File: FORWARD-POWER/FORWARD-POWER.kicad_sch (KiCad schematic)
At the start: 17 parts, among them J1 Conn_01x03_Pin, J2 Conn_01x03_Pin, J4 Screw_Terminal_01x04, U2 AMS1117-5.0, U3 AMS1117-3.3

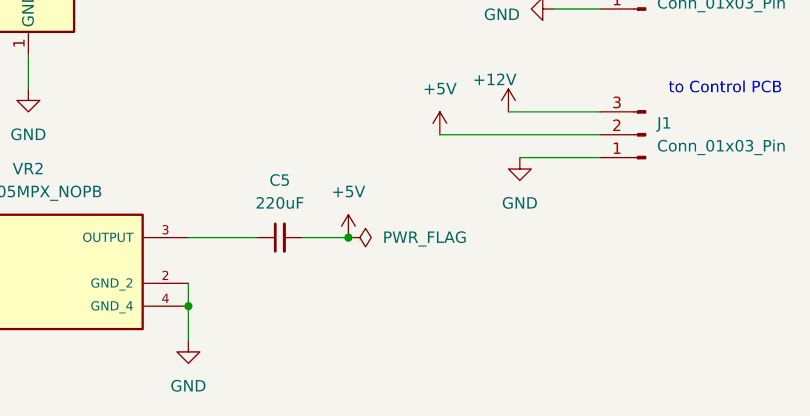
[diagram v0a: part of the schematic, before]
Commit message: ready to order (i think)
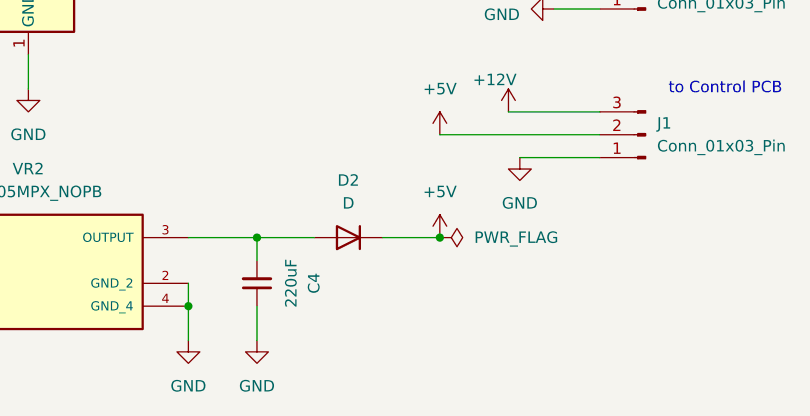
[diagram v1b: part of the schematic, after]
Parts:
- removed C5: 220uF, Capacitor_SMD:C_0805_2012Metric, symbol Device:C_Small
- added C4: 220uF, Capacitor_SMD:C_0805_2012Metric, symbol Device:C_Small
- added D2: D, Diode_SMD:D_0805_2012Metric, symbol Device:D
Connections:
- net +5V: now also D2.1 (K)
- net GND: now also C4.1
- net at VR2.3 (OUTPUT): now also C4.2, D2.2 (A)
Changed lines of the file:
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@@
+	)
+	(junction
+		(at 163.83 142.24)
+		(diameter 0)
+		(color 0 0 0 0)
 	)
 	(junction
@@
 	)
 	(junction
-		(at 173.99 142.24)
+		(at 184.15 142.24)
 		(diameter 0)
 		(color 0 0 0 0)
@@
 	(wire
 		(pts
-			(xy 173.99 142.24) (xy 168.91 142.24)
-		)
-		(stroke
-			(width 0)
-			(type default)
-		)
-	)
-	(wire
-		(pts
 			(xy 90.17 124.46) (xy 90.17 127)
 		)
@@
 	(wire
 		(pts
+			(xy 177.8 142.24) (xy 184.15 142.24)
+		)
+		(stroke
+			(width 0)
+			(type default)
+		)
+	)
+	(wire
+		(pts
 			(xy 123.19 72.39) (xy 132.08 72.39)
 		)
@@
 	(wire
 		(pts
+			(xy 163.83 142.24) (xy 163.83 144.78)
+		)
+		(stroke
+			(width 0)
+			(type default)
+		)
+	)
+	(wire
+		(pts
 			(xy 132.08 72.39) (xy 132.08 81.28)
 		)
@@
 	(wire
 		(pts
+			(xy 163.83 153.67) (xy 163.83 149.86)
+		)
+		(stroke
+			(width 0)
+			(type default)
+		)
+	)
+	(wire
+		(pts
 			(xy 156.21 149.86) (xy 156.21 147.32)
 		)
@@
 		(pts
 			(xy 156.21 153.67) (xy 156.21 149.86)
+		)
+		(stroke
+			(width 0)
+			(type default)
+		)
+	)
+	(wire
+		(pts
+			(xy 163.83 142.24) (xy 170.18 142.24)
 		)
 		(stroke
@@
 	)
 	(symbol
+		(lib_id "Device:D")
+		(at 173.99 142.24 180)
+		(unit 1)
+		(exclude_from_sim no)
+		(in_bom yes)
+		(on_board yes)
+		(dnp no)
+		(fields_autoplaced yes)
+		(property "Reference" "D2"
+			(at 173.99 135.89 0)
+			(effects
+				(font
+					(size 1.27 1.27)
+				)
+			)
+		)
+		(property "Value" "D"
+			(at 173.99 138.43 0)
+			(effects
+				(font
+					(size 1.27 1.27)
+				)
+			)
+		)
+		(property "Footprint" "Diode_SMD:D_0805_2012Metric"
+			(at 173.99 142.24 0)
+			(effects
+				(font
+					(size 1.27 1.27)
+				)
+				(hide yes)
+			)
+		)
+		(property "Datasheet" "~"
+			(at 173.99 142.24 0)
+			(effects
+				(font
+					(size 1.27 1.27)
+				)
+				(hide yes)
+			)
+		)
+		(property "Description" "Diode"
+			(at 173.99 142.24 0)
+			(effects
+				(font
+					(size 1.27 1.27)
+				)
+				(hide yes)
+			)
+		)
+		(property "Sim.Device" "D"
+			(at 173.99 142.24 0)
+			(effects
+				(font
+					(size 1.27 1.27)
+				)
+				(hide yes)
+			)
+		)
+		(property "Sim.Pins" "1=K 2=A"
+			(at 173.99 142.24 0)
+			(effects
+				(font
+					(size 1.27 1.27)
+				)
+				(hide yes)
+			)
+		)
+		(pin "1"
+		)
+		(pin "2"
+		)
+		(instances
+			(project ""
+				(path "/ce51f21b-ae90-4513-bbba-00af99e3d46b"
+					(reference "D2")
+					(unit 1)
+				)
+			)
+		)
+	)
+	(symbol
 		(lib_id "power:+6V")
 		(at 85.09 123.19 0)
@@
 	(symbol
 		(lib_id "power:PWR_FLAG")
-		(at 173.99 142.24 270)
+		(at 184.15 142.24 270)
 		(unit 1)
 		(exclude_from_sim no)
@@
 		(fields_autoplaced yes)
 		(property "Reference" "#FLG03"
-			(at 175.895 142.24 0)
+			(at 186.055 142.24 0)
 			(effects
 				(font
@@
 		)
 		(property "Value" "PWR_FLAG"
-			(at 177.8 142.2399 90)
+			(at 187.96 142.2399 90)
 			(effects
 				(font
@@
 		)
 		(property "Footprint" ""
-			(at 173.99 142.24 0)
+			(at 184.15 142.24 0)
 			(effects
 				(font
@@
 		)
 		(property "Datasheet" "~"
-			(at 173.99 142.24 0)
+			(at 184.15 142.24 0)
 			(effects
 				(font
@@
 		)
 		(property "Description" "Special symbol for telling ERC where power comes from"
-			(at 173.99 142.24 0)
+			(at 184.15 142.24 0)
 			(effects
 				(font
@@
 	)
 	(symbol
-		(lib_id "Device:C_Small")
-		(at 166.37 142.24 90)
-		(unit 1)
-		(exclude_from_sim no)
-		(in_bom yes)
-		(on_board yes)
-		(dnp no)
-		(fields_autoplaced yes)
-		(property "Reference" "C5"
-			(at 166.3763 135.89 90)
-			(effects
-				(font
-					(size 1.27 1.27)
-				)
-			)
-		)
-		(property "Value" "220uF"
-			(at 166.3763 138.43 90)
-			(effects
-				(font
-					(size 1.27 1.27)
-				)
-			)
-		)
-		(property "Footprint" "Capacitor_SMD:C_0805_2012Metric"
-			(at 166.37 142.24 0)
-			(effects
-				(font
-					(size 1.27 1.27)
-				)
-				(hide yes)
-			)
-		)
-		(property "Datasheet" "~"
-			(at 166.37 142.24 0)
-			(effects
-				(font
-					(size 1.27 1.27)
-				)
-				(hide yes)
-			)
-		)
-		(property "Description" "Unpolarized capacitor, small symbol"
-			(at 166.37 142.24 0)
-			(effects
-				(font
-					(size 1.27 1.27)
-				)
-				(hide yes)
-			)
-		)
-		(pin "2"
-		)
-		(pin "1"
-		)
-		(instances
-			(project ""
-				(path "/ce51f21b-ae90-4513-bbba-00af99e3d46b"
-					(reference "C5")
-					(unit 1)
-				)
-			)
-		)
-	)
-	(symbol
 		(lib_id "power:+3.3V")
 		(at 196.85 111.76 90)
@@
 	)
 	(symbol
+		(lib_id "power:GND")
+		(at 163.83 153.67 0)
+		(unit 1)
+		(exclude_from_sim no)
+		(in_bom yes)
+		(on_board yes)
+		(dnp no)
+		(fields_autoplaced yes)
+		(property "Reference" "#PWR06"
+			(at 163.83 160.02 0)
+			(effects
+				(font
+					(size 1.27 1.27)
+				)
+				(hide yes)
+			)
+		)
+		(property "Value" "GND"
+			(at 163.83 158.75 0)
+			(effects
+				(font
+					(size 1.27 1.27)
+				)
+			)
+		)
+		(property "Footprint" ""
+			(at 163.83 153.67 0)
+			(effects
+				(font
+					(size 1.27 1.27)
+				)
+				(hide yes)
+			)
+		)
+		(property "Datasheet" ""
+			(at 163.83 153.67 0)
+			(effects
+				(font
+					(size 1.27 1.27)
+				)
+				(hide yes)
+			)
+		)
+		(property "Description" ""
+			(at 163.83 153.67 0)
+			(effects
+				(font
+					(size 1.27 1.27)
+				)
+				(hide yes)
+			)
+		)
+		(pin "1"
+		)
+		(instances
+			(project "FORWARD-POWER"
+				(path "/ce51f21b-ae90-4513-bbba-00af99e3d46b"
+					(reference "#PWR06")
+					(unit 1)
+				)
+			)
+		)
+	)
+	(symbol
 		(lib_id "power:PWR_FLAG")
 		(at 163.83 114.3 0)
@@
 	)
 	(symbol
+		(lib_id "Device:C_Small")
+		(at 163.83 147.32 0)
+		(mirror x)
+		(unit 1)
+		(exclude_from_sim no)
+		(in_bom yes)
+		(on_board yes)
+		(dnp no)
+		(property "Reference" "C4"
+			(at 170.18 147.3137 90)
+			(effects
+				(font
+					(size 1.27 1.27)
+				)
+			)
+		)
+		(property "Value" "220uF"
+			(at 167.64 147.3137 90)
+			(effects
+				(font
+					(size 1.27 1.27)
+				)
+			)
+		)
+		(property "Footprint" "Capacitor_SMD:C_0805_2012Metric"
+			(at 163.83 147.32 0)
+			(effects
+				(font
+					(size 1.27 1.27)
+				)
+				(hide yes)
+			)
+		)
+		(property "Datasheet" "~"
+			(at 163.83 147.32 0)
+			(effects
+				(font
+					(size 1.27 1.27)
+				)
+				(hide yes)
+			)
+		)
+		(property "Description" "Unpolarized capacitor, small symbol"
+			(at 163.83 147.32 0)
+			(effects
+				(font
+					(size 1.27 1.27)
+				)
+				(hide yes)
+			)
+		)
+		(pin "2"
+		)
+		(pin "1"
+		)
+		(instances
+			(project "FORWARD-POWER"
+				(path "/ce51f21b-ae90-4513-bbba-00af99e3d46b"
+					(reference "C4")
+					(unit 1)
+				)
+			)
+		)
+	)
+	(symbol
 		(lib_id "Mechanical:MountingHole")
 		(at 190.5 81.28 0)
@@
 	(symbol
 		(lib_id "power:+5V")
-		(at 173.99 142.24 0)
+		(at 184.15 142.24 0)
 		(unit 1)
 		(exclude_from_sim no)
@@
 		(fields_autoplaced yes)
 		(property "Reference" "#PWR012"
-			(at 173.99 146.05 0)
+			(at 184.15 146.05 0)
 			(effects
 				(font
@@
 		)
 		(property "Value" "+5V"
-			(at 173.99 137.16 0)
+			(at 184.15 137.16 0)
 			(effects
 				(font
@@
 		)
 		(property "Footprint" ""
-			(at 173.99 142.24 0)
+			(at 184.15 142.24 0)
 			(effects
 				(font
@@
 		)
 		(property "Datasheet" ""
-			(at 173.99 142.24 0)
+			(at 184.15 142.24 0)
 			(effects
 				(font
@@
 		)
 		(property "Description" ""
-			(at 173.99 142.24 0)
-			(effects
-				(font
+			(at 184.15 142.24 0)
+			(effects
+				(font
